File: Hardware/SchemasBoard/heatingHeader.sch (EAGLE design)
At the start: 30 parts, among them IC1 DS1820

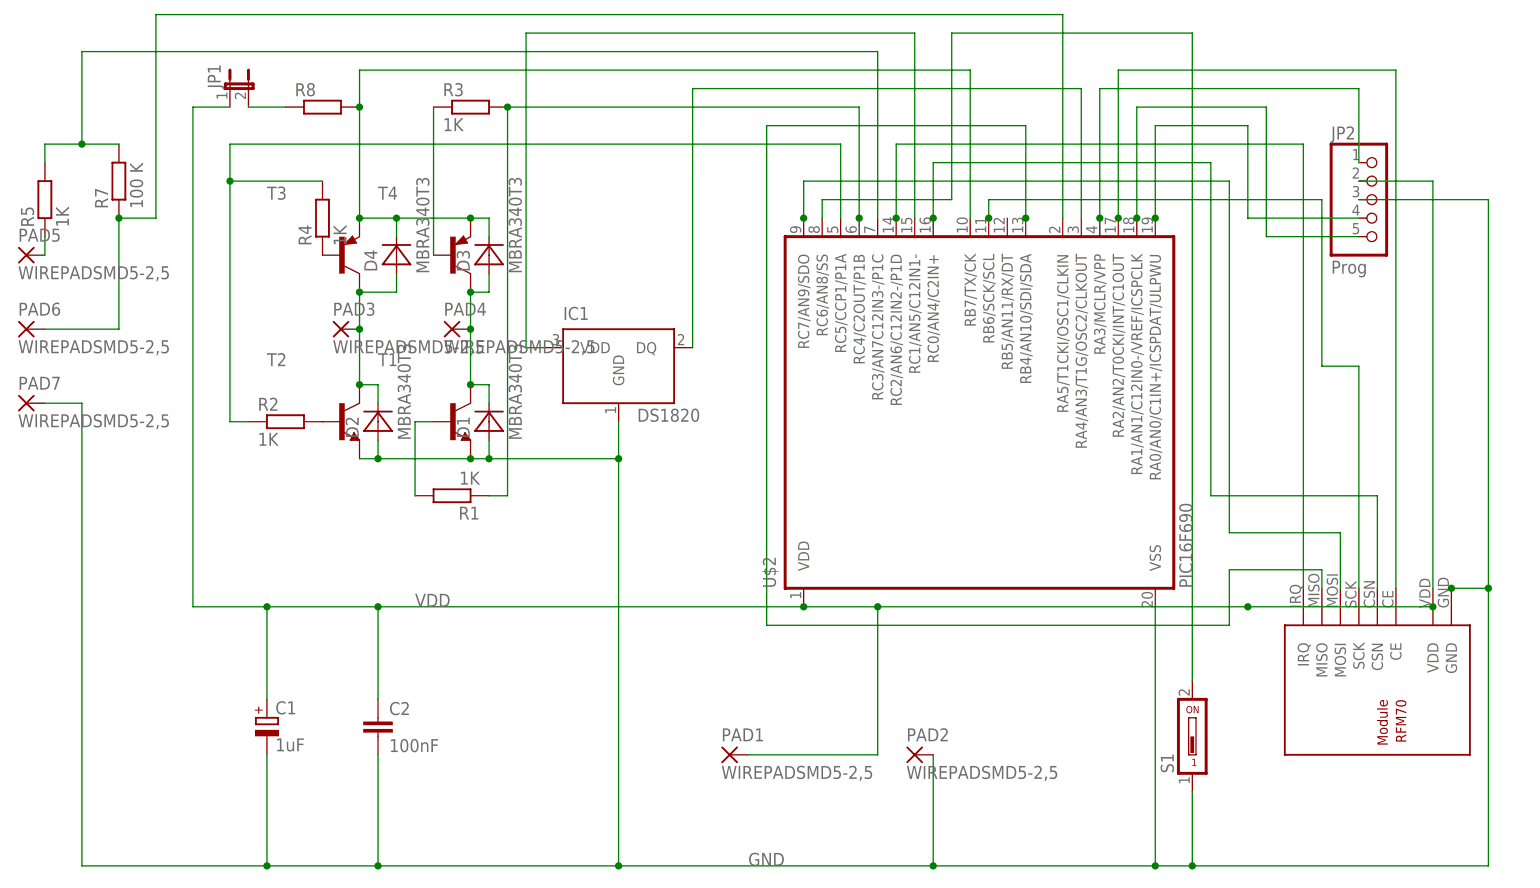
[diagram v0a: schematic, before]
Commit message: a
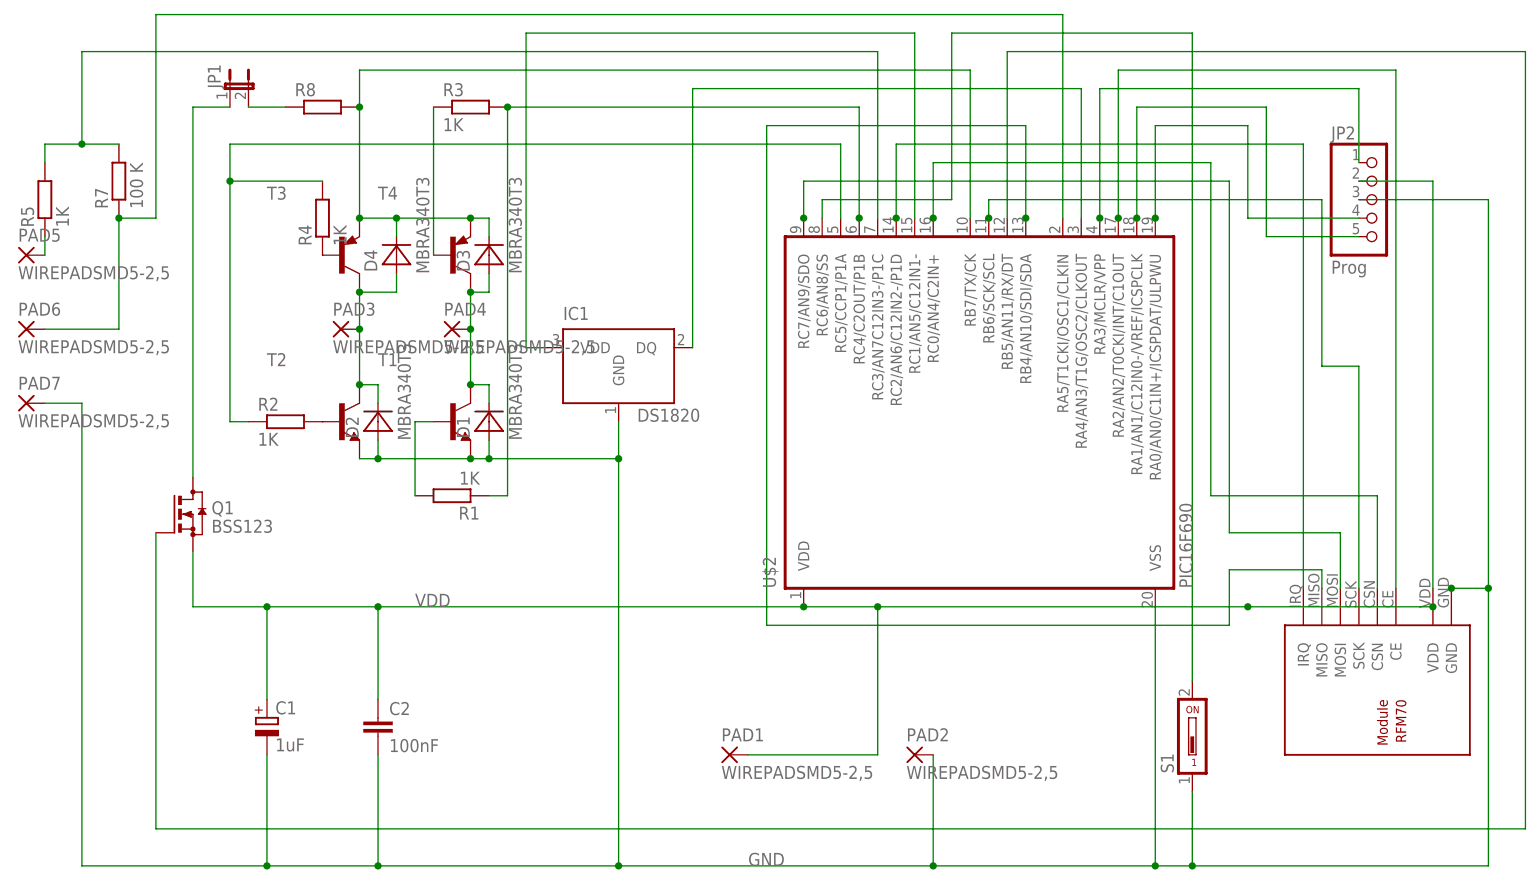
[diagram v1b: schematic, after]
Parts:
- added Q1: BSS123, transistor-small-signal:BSS123
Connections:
- new net N$11: JP1.1, Q1.D
- new net N$28: Q1.G, U$2.RB5/AN11/RX/DT
- net VDD: now also Q1.S; no longer JP1.1
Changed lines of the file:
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@@
 <part name="C1" library="resistor" deviceset="CPOL-EU" device="SMCA" value="1uF"/>
 <part name="C2" library="resistor" deviceset="C-EU" device="C2012" value="100nF"/>
+<part name="Q1" library="transistor-small-signal" deviceset="BSS123" device=""/>
 </parts>
 <sheets>
@@
 <instance part="C1" gate="G$1" x="10.16" y="50.8"/>
 <instance part="C2" gate="G$1" x="25.4" y="50.8"/>
+<instance part="Q1" gate="G$1" x="0" y="78.74"/>
 </instances>
 <busses>
@@
 <segment>
 <pinref part="U$2" gate="G$1" pin="VDD"/>
-<wire x1="0" y1="134.62" x2="0" y2="66.04" width="0.1524" layer="91"/>
 <wire x1="83.82" y1="66.04" x2="93.98" y2="66.04" width="0.1524" layer="91"/>
 <wire x1="93.98" y1="66.04" x2="144.78" y2="66.04" width="0.1524" layer="91"/>
@@
 <wire x1="10.16" y1="66.04" x2="25.4" y2="66.04" width="0.1524" layer="91"/>
 <wire x1="25.4" y1="66.04" x2="83.82" y2="66.04" width="0.1524" layer="91"/>
-<wire x1="0" y1="134.62" x2="5.08" y2="134.62" width="0.1524" layer="91"/>
-<pinref part="JP1" gate="A" pin="1"/>
 <label x="30.48" y="66.04" size="1.778" layer="95"/>
 <pinref part="C1" gate="G$1" pin="+"/>
@@
 <junction x="25.4" y="66.04"/>
 <junction x="170.18" y="66.04"/>
+<pinref part="Q1" gate="G$1" pin="S"/>
+<wire x1="0" y1="66.04" x2="0" y2="73.66" width="0.1524" layer="91"/>
 </segment>
 <segment>
@@
 </segment>
 </net>
+<net name="N$11" class="0">
+<segment>
+<pinref part="JP1" gate="A" pin="1"/>
+<wire x1="0" y1="134.62" x2="5.08" y2="134.62" width="0.1524" layer="91"/>
+<pinref part="Q1" gate="G$1" pin="D"/>
+<wire x1="0" y1="83.82" x2="0" y2="134.62" width="0.1524" layer="91"/>
+</segment>
+</net>
+<net name="N$28" class="0">
+<segment>
+<pinref part="U$2" gate="G$1" pin="RB5/AN11/RX/DT"/>
+<wire x1="111.76" y1="119.38" x2="111.76" y2="142.24" width="0.1524" layer="91"/>
+<wire x1="111.76" y1="142.24" x2="182.88" y2="142.24" width="0.1524" layer="91"/>
+<wire x1="182.88" y1="142.24" x2="182.88" y2="35.56" width="0.1524" layer="91"/>
+<pinref part="Q1" gate="G$1" pin="G"/>
+<wire x1="182.88" y1="35.56" x2="-5.08" y2="35.56" width="0.1524" layer="91"/>
+<wire x1="-5.08" y1="35.56" x2="-5.08" y2="76.2" width="0.1524" layer="91"/>
+</segment>
+</net>
